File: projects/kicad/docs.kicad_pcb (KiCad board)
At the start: 2 copper layers, 17 parts, among them SW1 SW_PUSH, SW2 SW_PUSH, SW3 SW_PUSH, SW4 SW_PUSH, SW5 SW_PUSH, SW6 SW_PUSH, SW7 RotaryEncoder_Switch, U2 LCD

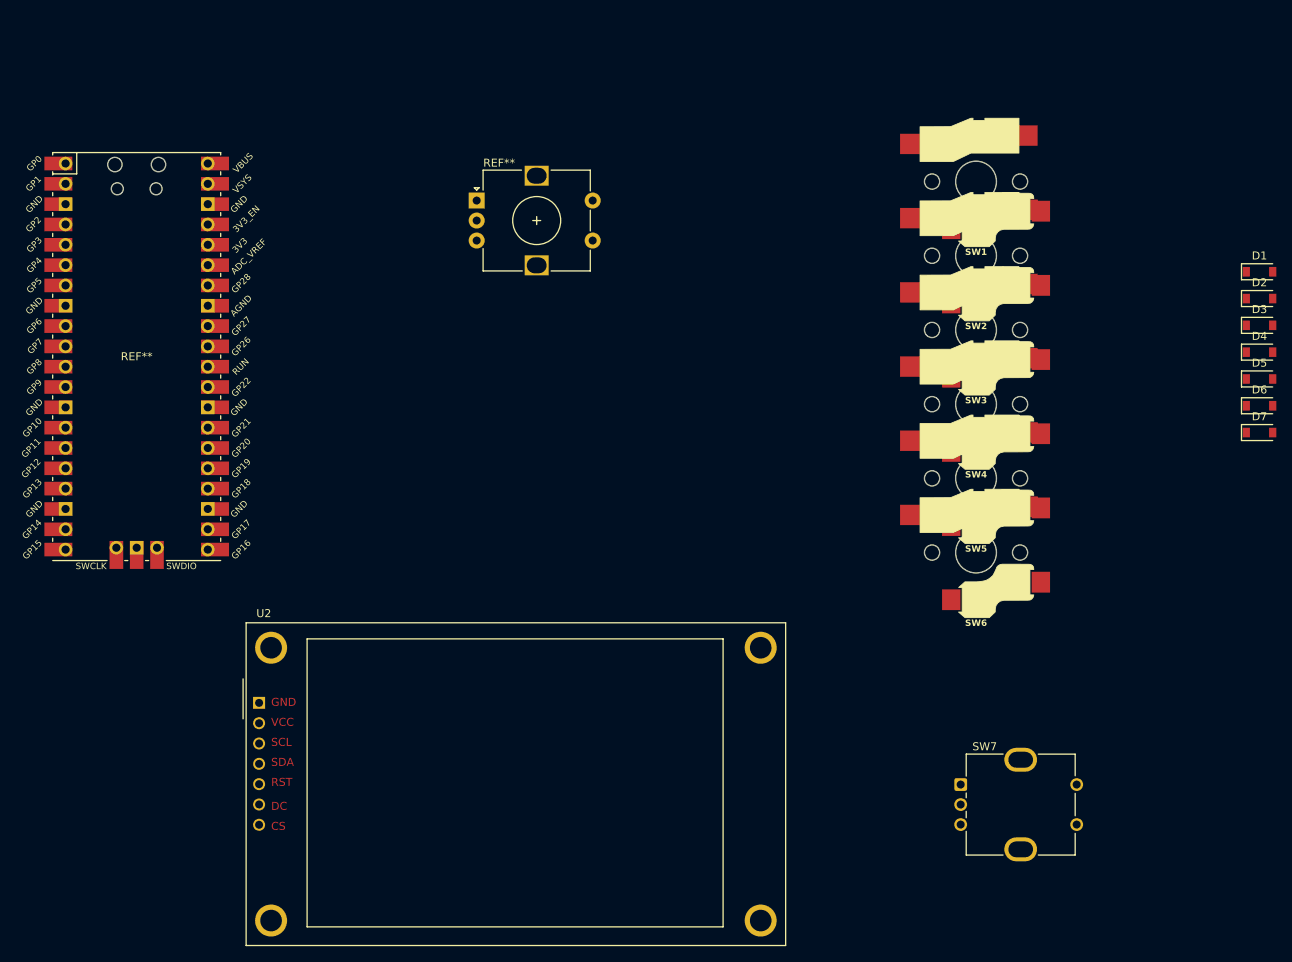
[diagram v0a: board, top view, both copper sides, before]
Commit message: chocolate: Update_0126
とりあえず部品の配置。
配線はまだ手つけてないです。。
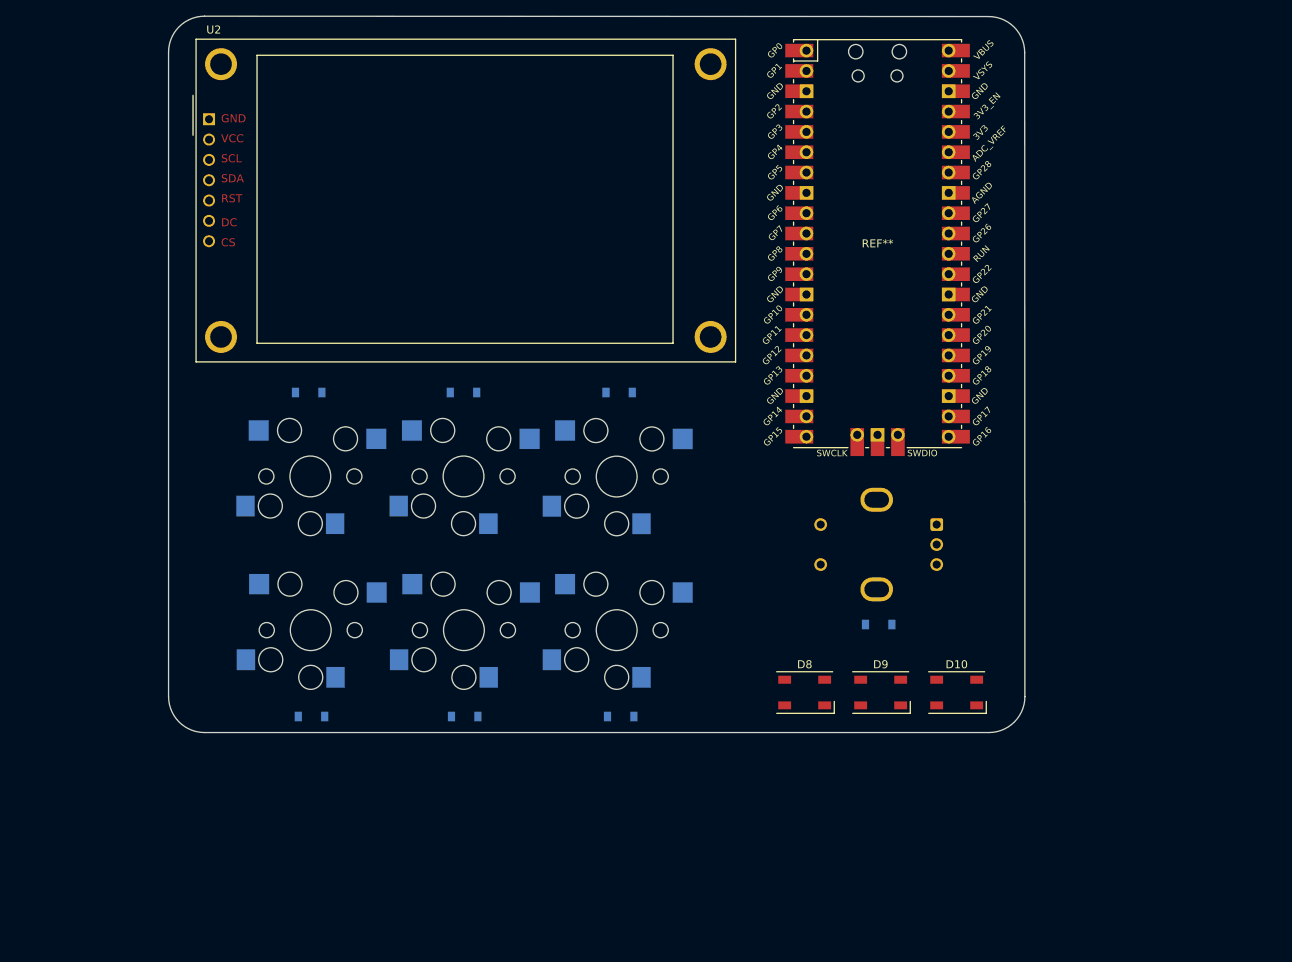
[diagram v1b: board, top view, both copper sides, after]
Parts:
- removed the REF** at (126.0, 46.5)
- added D10: LED, kbd:LED_WS2812B-PLCC4, F.Cu at (186.0, 108.0)
- added D8: LED, kbd:LED_WS2812B-PLCC4, F.Cu at (167.0, 108.0)
- added D9: LED, kbd:LED_WS2812B-PLCC4, F.Cu at (176.5, 108.0)
- D1, D2, D3, D4, D5, D6, D7, SW1, SW2, SW3, SW4, SW5, SW6, SW7: moved to B.Cu
- moved D2 129.5 mm to (105.3, 111.0), turned to 180 degrees
- moved D1 119.8 mm to (105.0, 70.5), turned to 180 degrees
- moved D4 109.3 mm to (124.5, 111.0), turned to 180 degrees
- moved D3 99.9 mm to (124.3, 70.5), turned to 180 degrees
- moved SW2 95.4 mm to (105.3, 100.2), turned to 180 degrees
- moved REF** 93.7 mm to (176.1, 51.9)
- moved SW1 91.0 mm to (105.2, 81.0), turned to 180 degrees
- moved D6 88.8 mm to (144.0, 111.0), turned to 180 degrees
- moved D5 80.1 mm to (143.8, 70.5), turned to 180 degrees
- moved U2 73.2 mm to (92.5, 36.3)
- moved SW4 70.0 mm to (124.4, 100.2), turned to 180 degrees
- moved SW3 66.6 mm to (124.4, 81.0), turned to 180 degrees
- moved D7 53.3 mm to (176.2, 99.5), turned to 180 degrees
- moved SW6 46.0 mm to (143.5, 100.2), turned to 180 degrees
- moved SW5 44.9 mm to (143.5, 81.0), turned to 180 degrees
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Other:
- board outline added: 107 x 89.5 mm
